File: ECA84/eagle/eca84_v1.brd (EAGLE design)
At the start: 223 x 127 mm, 186 parts

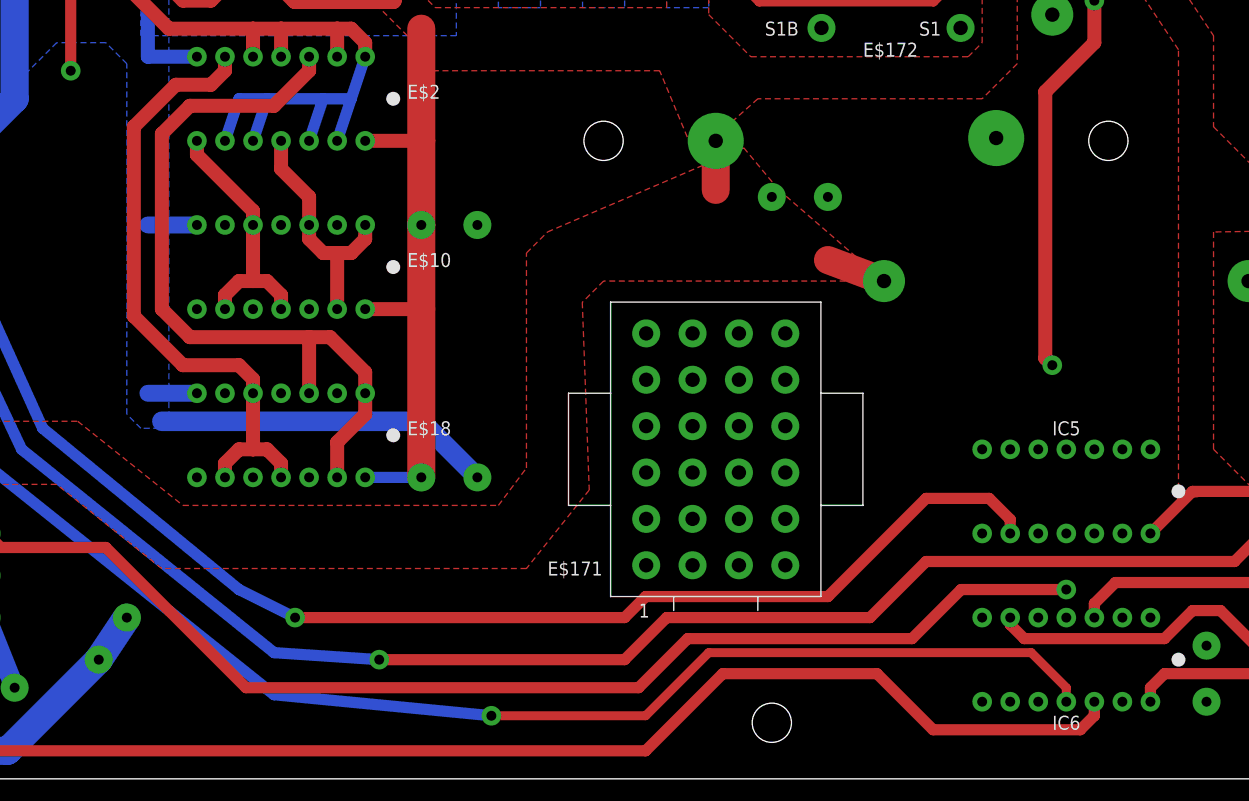
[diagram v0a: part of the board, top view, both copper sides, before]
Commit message: Antes de cambiar angulo de pistas
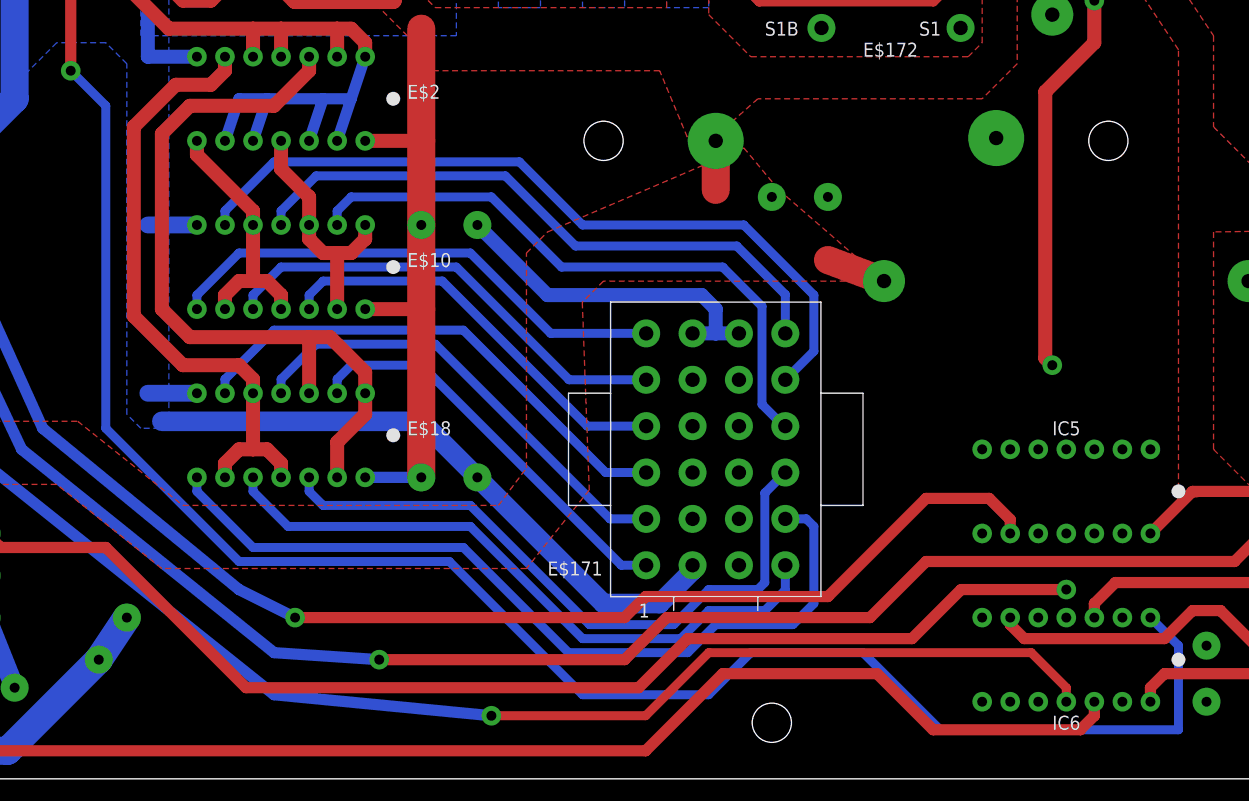
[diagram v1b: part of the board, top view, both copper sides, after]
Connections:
- new net S$80: E$10.P$6, E$171.P$20
- new net S$81: E$10.P$4, E$171.P$24
- new net S$82: E$10.P$2, E$171.P$16
- new net S$83: E$10.P$10, E$171.P$17
- new net S$84: E$10.P$12, E$171.P$13
- new net S$85: E$10.P$8, E$171.P$21
- new net S$86: E$171.P$12, E$18.P$12
- new net S$87: E$171.P$9, E$18.P$6
- new net S$88: E$171.P$5, E$18.P$4
- new net S$89: E$171.P$1, E$18.P$2
- new net S$90: E$171.P$4, E$18.P$10
- new net S$91: E$171.P$8, E$18.P$8
- net GND: now also E$171.P$10, E$171.P$11, E$171.P$14, E$171.P$15, E$171.P$18, E$171.P$19, E$171.P$2, E$171.P$22, E$171.P$23, E$171.P$3, E$171.P$6, E$171.P$7, E$94.P$1
- net S$69: now also IC15.P$2, IC6.P$1
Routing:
- net S$69: track 78.7 -> 235.2 mm
- net S$91: track 0.00 -> 74.9 mm
- net S$80: track 0.00 -> 70.2 mm
- net S$86: track 0.00 -> 59.9 mm
- net S$90: track 0.00 -> 59.1 mm
- net GND: track 271.3 -> 328.4 mm
- net S$81: track 0.00 -> 56.2 mm
- net S$82: track 0.00 -> 56.2 mm
- net S$87: track 0.00 -> 46.6 mm
- net S$85: track 0.00 -> 46.6 mm
- net S$88: track 0.00 -> 42.2 mm
- net S$83: track 0.00 -> 42.2 mm
- net S$84: track 0.00 -> 37.8 mm
- net S$89: track 0.00 -> 37.3 mm
